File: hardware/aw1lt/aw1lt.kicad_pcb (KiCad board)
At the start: 2 copper layers, 30 x 22 mm, 27 parts, among them J1 ISP_FTDI, Q1 Q_NPN_CBE, SW1 SW_Push, SW2 SW_Push, SW3 SW_Push, U1 DS3231MZ, U2 ATMEGA328P-AU

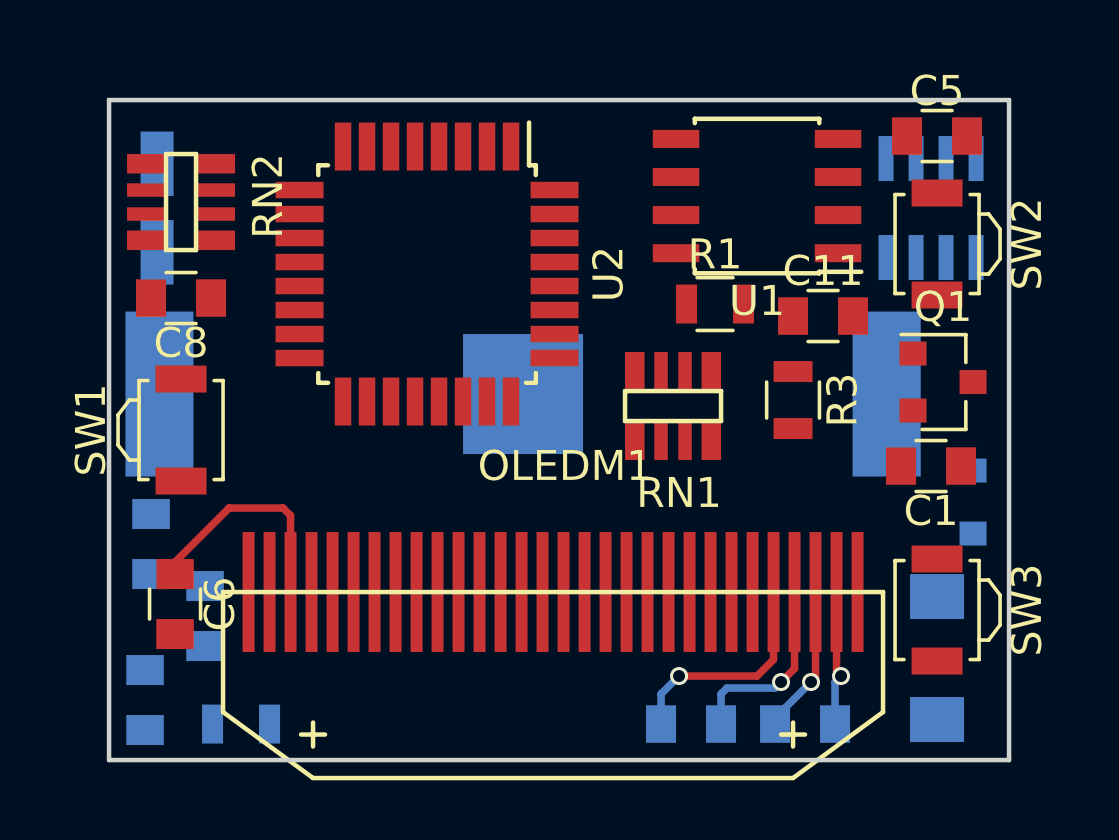
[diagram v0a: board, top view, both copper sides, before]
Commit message: working on routing
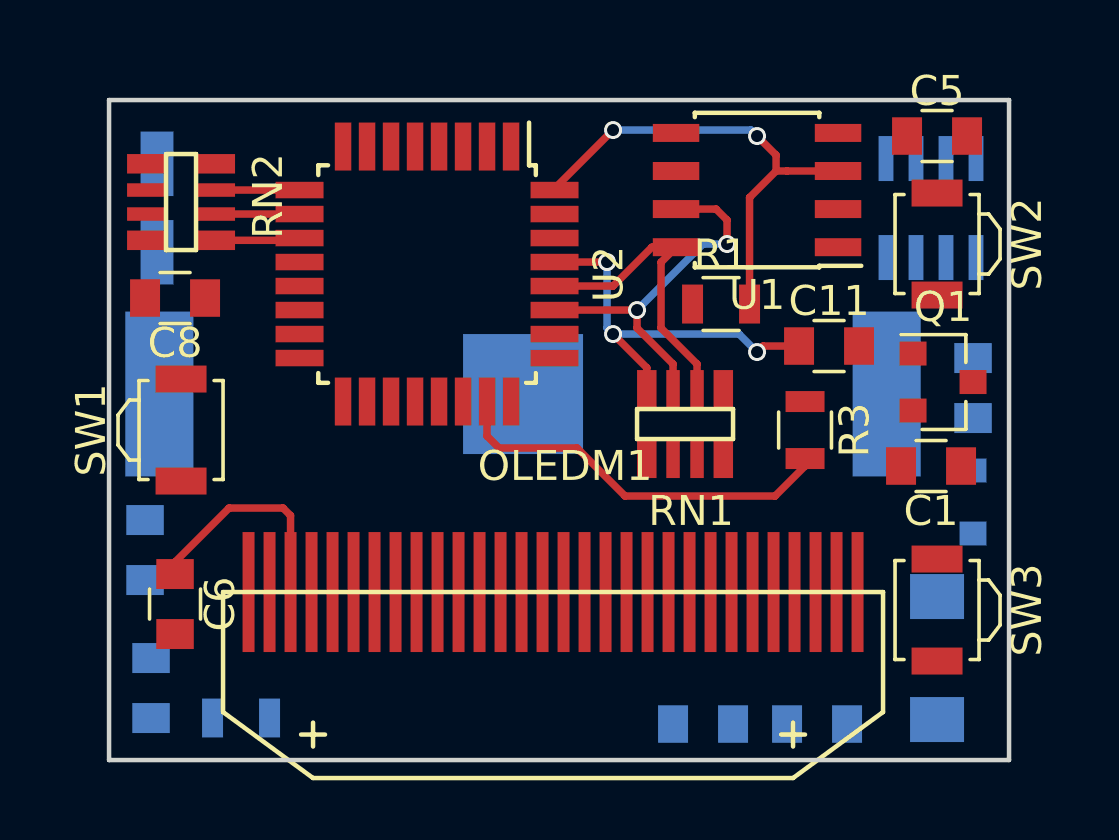
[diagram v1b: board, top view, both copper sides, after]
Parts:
- moved C4 26.7 mm to (153.8, 134.6)
- moved R3 1.08 mm to (148.2, 136.0)
- moved C11 1.02 mm to (149.0, 133.2)
- moved RN1 0.72 mm to (144.2, 135.8)
- moved C7 0.45 mm to (126.4, 144.6)
- moved C2 0.40 mm to (144.8, 145.8)
- moved C3 0.40 mm to (148.6, 145.8)
- moved C10 0.28 mm to (126.2, 140.0)
- moved R1 0.20 mm to (145.4, 131.8)
- moved R2 0.20 mm to (129.4, 145.6)
- moved C8 0.20 mm to (127.2, 131.6)
- moved U1 0.20 mm to (146.6, 128.0)
- turned C9 to 90 degrees
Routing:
- net INT0: track 0.00 -> 16.0 mm, vias 0 -> 2
- net SPKR: track 0.00 -> 13.2 mm
- net Net-(C11-Pad1): track 0.00 -> 13.1 mm, vias 0 -> 3
- net SDA: track 0.00 -> 12.5 mm, vias 0 -> 2
- net SCL: track 0.00 -> 10.0 mm
- net Net-(C2-Pad2): track 7.48 -> 0.00 mm, vias 1 -> 0
- net Net-(C2-Pad1): track 6.35 -> 0.00 mm, vias 1 -> 0
- net Net-(C3-Pad2): track 4.96 -> 0.00 mm, vias 1 -> 0
- net Net-(C3-Pad1): track 4.54 -> 0.00 mm, vias 1 -> 0
- net PB2: track 0.11 -> 2.94 mm
- net PB1: track 0.00 -> 2.80 mm
- net PB0: track 0.00 -> 2.80 mm
